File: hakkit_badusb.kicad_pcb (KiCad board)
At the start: 2 copper layers, 16.4 x 42.8 mm, 20 parts, among them J1 USB3_A, U1 RP2040, U2 W25Q128JVP, U3 LT1962-3.3, Y1 12MHz Cryst

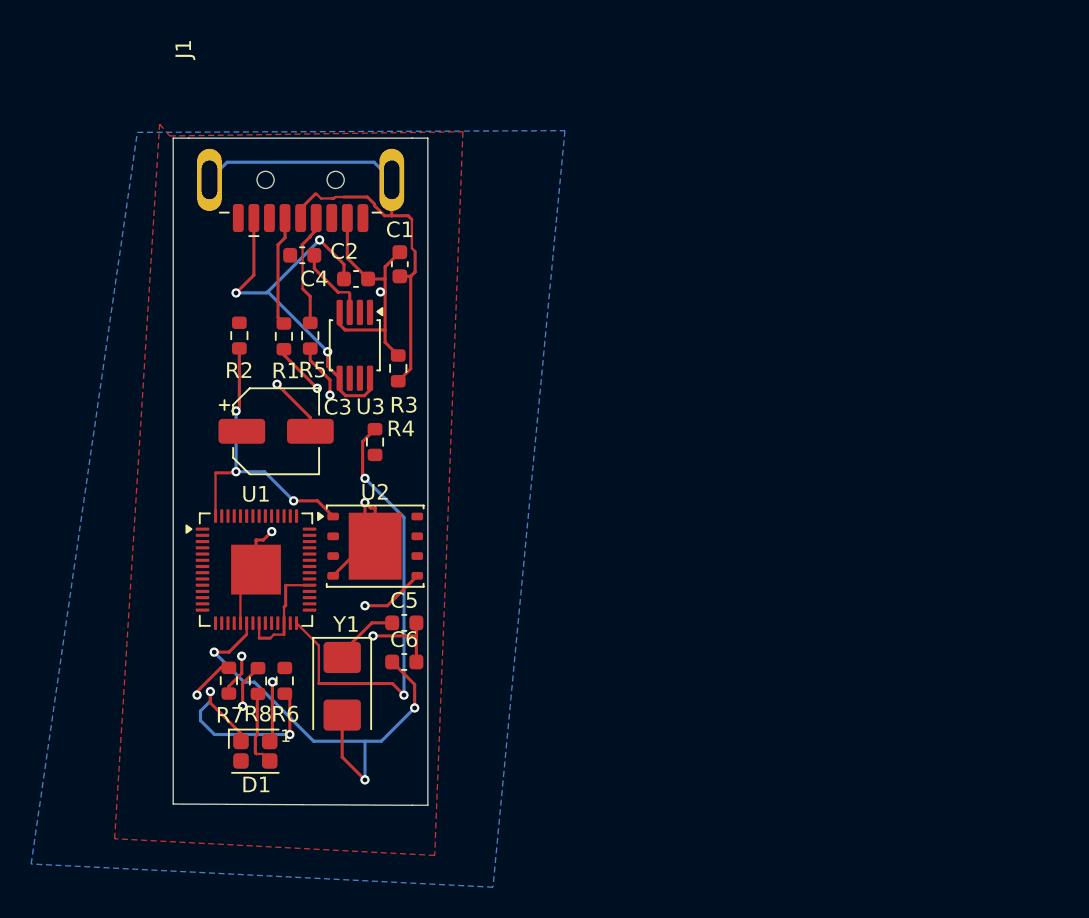
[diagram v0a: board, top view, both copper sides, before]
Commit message: remade pcb
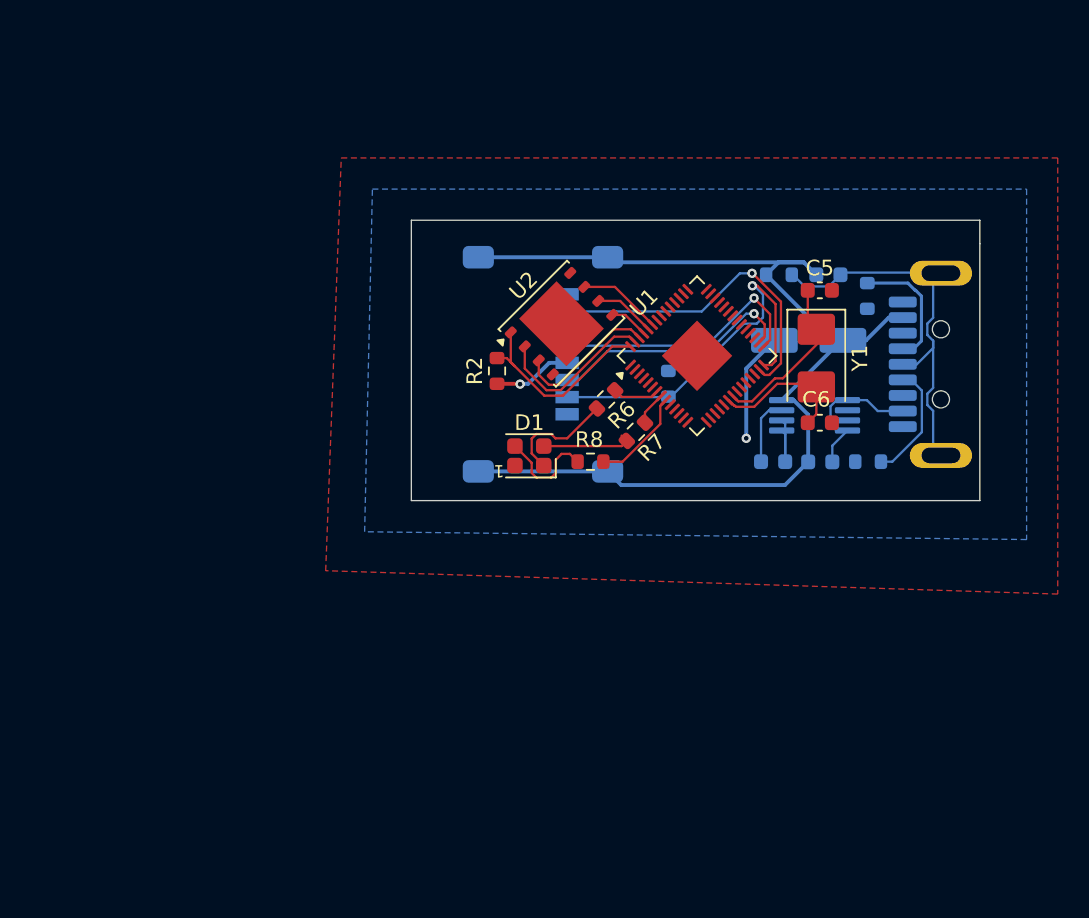
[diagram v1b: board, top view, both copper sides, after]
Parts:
- added J2: Micro_SD_Card, Connector_Card:microSD_HC_Molex_47219-2001, B.Cu at (112.4, 45.8)
- C1, C2, C3, C4, J1, R1, R3, R4, R5, U3: moved to B.Cu
- moved J1 53.5 mm to (146.9, 45.8), turned to 0 degrees
- moved R1 38.4 mm to (133.8, 52.0), turned to 180 degrees
- moved Y1 37.0 mm to (130.5, 45.4)
- moved R5 35.9 mm to (133.8, 41.4)
- moved C3 34.7 mm to (130.0, 44.2)
- moved C5 34.2 mm to (130.7, 41.0)
- moved C2 33.0 mm to (127.7, 52.0), turned to 180 degrees
- moved C4 32.0 mm to (130.8, 52.0), turned to 180 degrees
- moved U1 31.5 mm to (122.8, 45.2), turned to 45 degrees
- moved C6 30.8 mm to (130.7, 49.5)
- moved R7 30.6 mm to (118.9, 50.1), turned to -135 degrees
- moved U3 29.9 mm to (130.4, 49.0), turned to 0 degrees
- moved C1 27.5 mm to (131.3, 40.0), turned to 180 degrees
- moved R6 27.4 mm to (117.0, 48.0), turned to -135 degrees
- moved D1 25.9 mm to (112.1, 51.6), turned to 180 degrees
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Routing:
- net GND: track 46.4 -> 68.8 mm, vias 6 -> 0
- net /SD_MISO: track 0.00 -> 21.3 mm, vias 0 -> 1
- net Net-(U1-XIN): track 30.2 -> 9.06 mm, vias 3 -> 0
- net /SD_SCK: track 0.00 -> 17.0 mm, vias 0 -> 1
- net +3V3: track 0.00 -> 16.9 mm, vias 0 -> 2
- net +5V: track 26.4 -> 9.92 mm, vias 3 -> 0
- net /SD_MOSI: track 0.00 -> 16.0 mm, vias 0 -> 1
- net Net-(U1-QSPI_SD1): track 0.00 -> 10.6 mm
- net Net-(U1-QSPI_SD2): track 0.00 -> 9.35 mm
- net Net-(J1-DRAIN): track 35.5 -> 26.2 mm
- net Net-(D1-RA): track 15.0 -> 7.27 mm, vias 2 -> 0
- net Net-(U1-RUN): track 7.41 -> 0.00 mm
- net Net-(U1-XOUT): track 4.31 -> 10.7 mm
- net Net-(U1-~{QSPI_SS}): track 19.5 -> 13.1 mm, vias 3 -> 0
- net Net-(U1-QSPI_SD3): track 0.00 -> 5.39 mm
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- added copper zone on B.Cu, net +3V3
- added copper zone on F.Cu, net GND
- removed copper zone on F.Cu, net +3V3
- removed copper zone on B.Cu, net GND
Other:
- board size 16.4 x 42.8 mm -> 36.5 x 18 mm
